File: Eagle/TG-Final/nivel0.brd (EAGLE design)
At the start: 21 parts

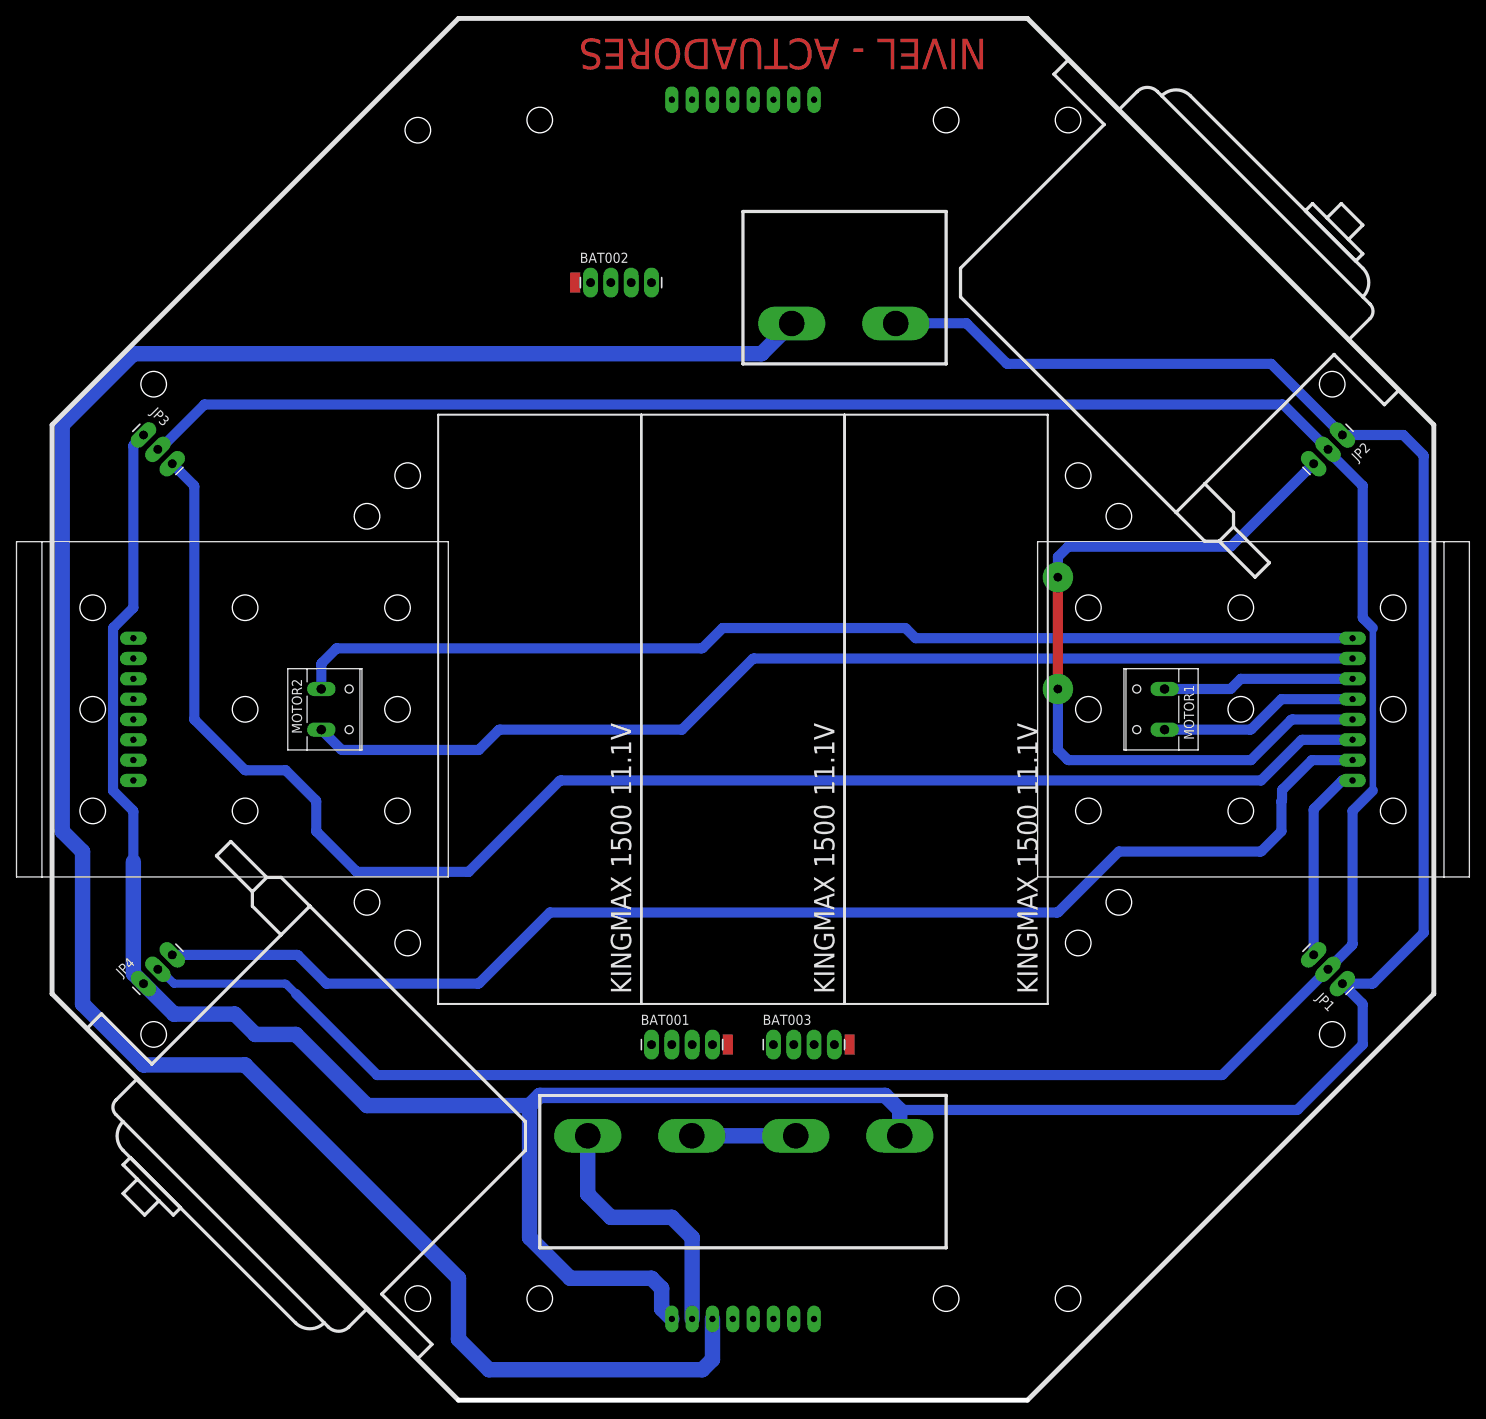
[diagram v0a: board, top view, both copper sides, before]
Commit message: Routing placa Actuadores. Listo??
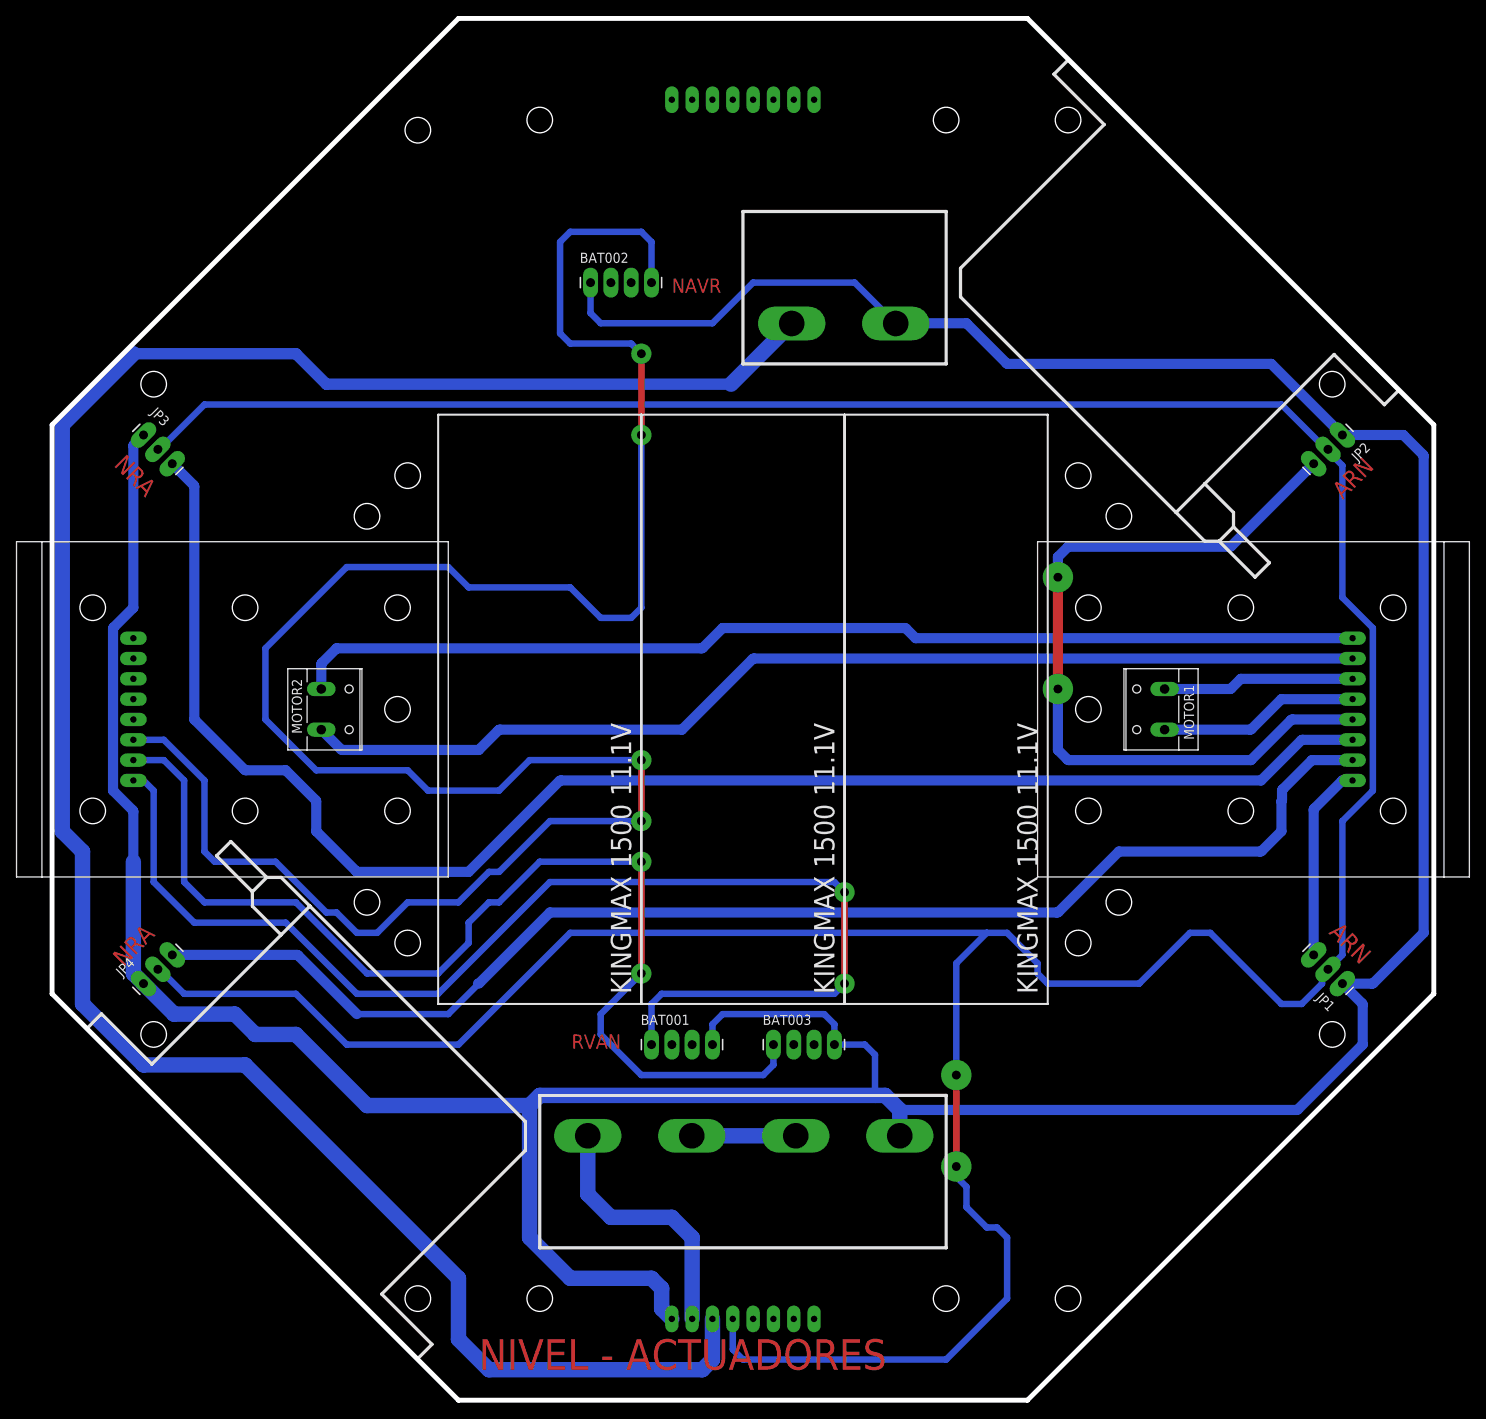
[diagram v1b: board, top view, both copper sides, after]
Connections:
- removed net +6V: JP1.2, JP2.2, JP3.2, JP4.2
- new net P$1: JP1.2, JP2.2, JP3.2, JP4.2, U$1.PIN19
- new net SENSE1: BAT001.1, U$1.PIN15
- new net SENSE2: BAT002.4, U$1.PIN13
- new net SENSE3: BAT003.1, U$1.PIN14
- net VSS: now also BAT001.4, BAT002.1, BAT003.4
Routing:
- net P$1: track 0.00 -> 481.1 mm, vias 0 -> 2
- net +6V: track 377.6 -> 0.00 mm
- net SENSE2: track 0.00 -> 279.6 mm, vias 0 -> 4
- net SENSE1: track 0.00 -> 154.6 mm, vias 0 -> 2
- net SENSE3: track 0.00 -> 139.7 mm, vias 0 -> 2
- net VSS: track 432.2 -> 511.0 mm
- net +12V: track 277.6 -> 281.0 mm
- net SERVO04: track 163.5 -> 166.7 mm
- added copper zone on layer 16, net N$2
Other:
- board outline added: 172.7 x 172.7 mm
- board text added: "ARN"
- board text added: "NAVR"
- board text added: "NRA"
- board text added: "RVAN"

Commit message: Mejoras en placa de Actuadores y otros
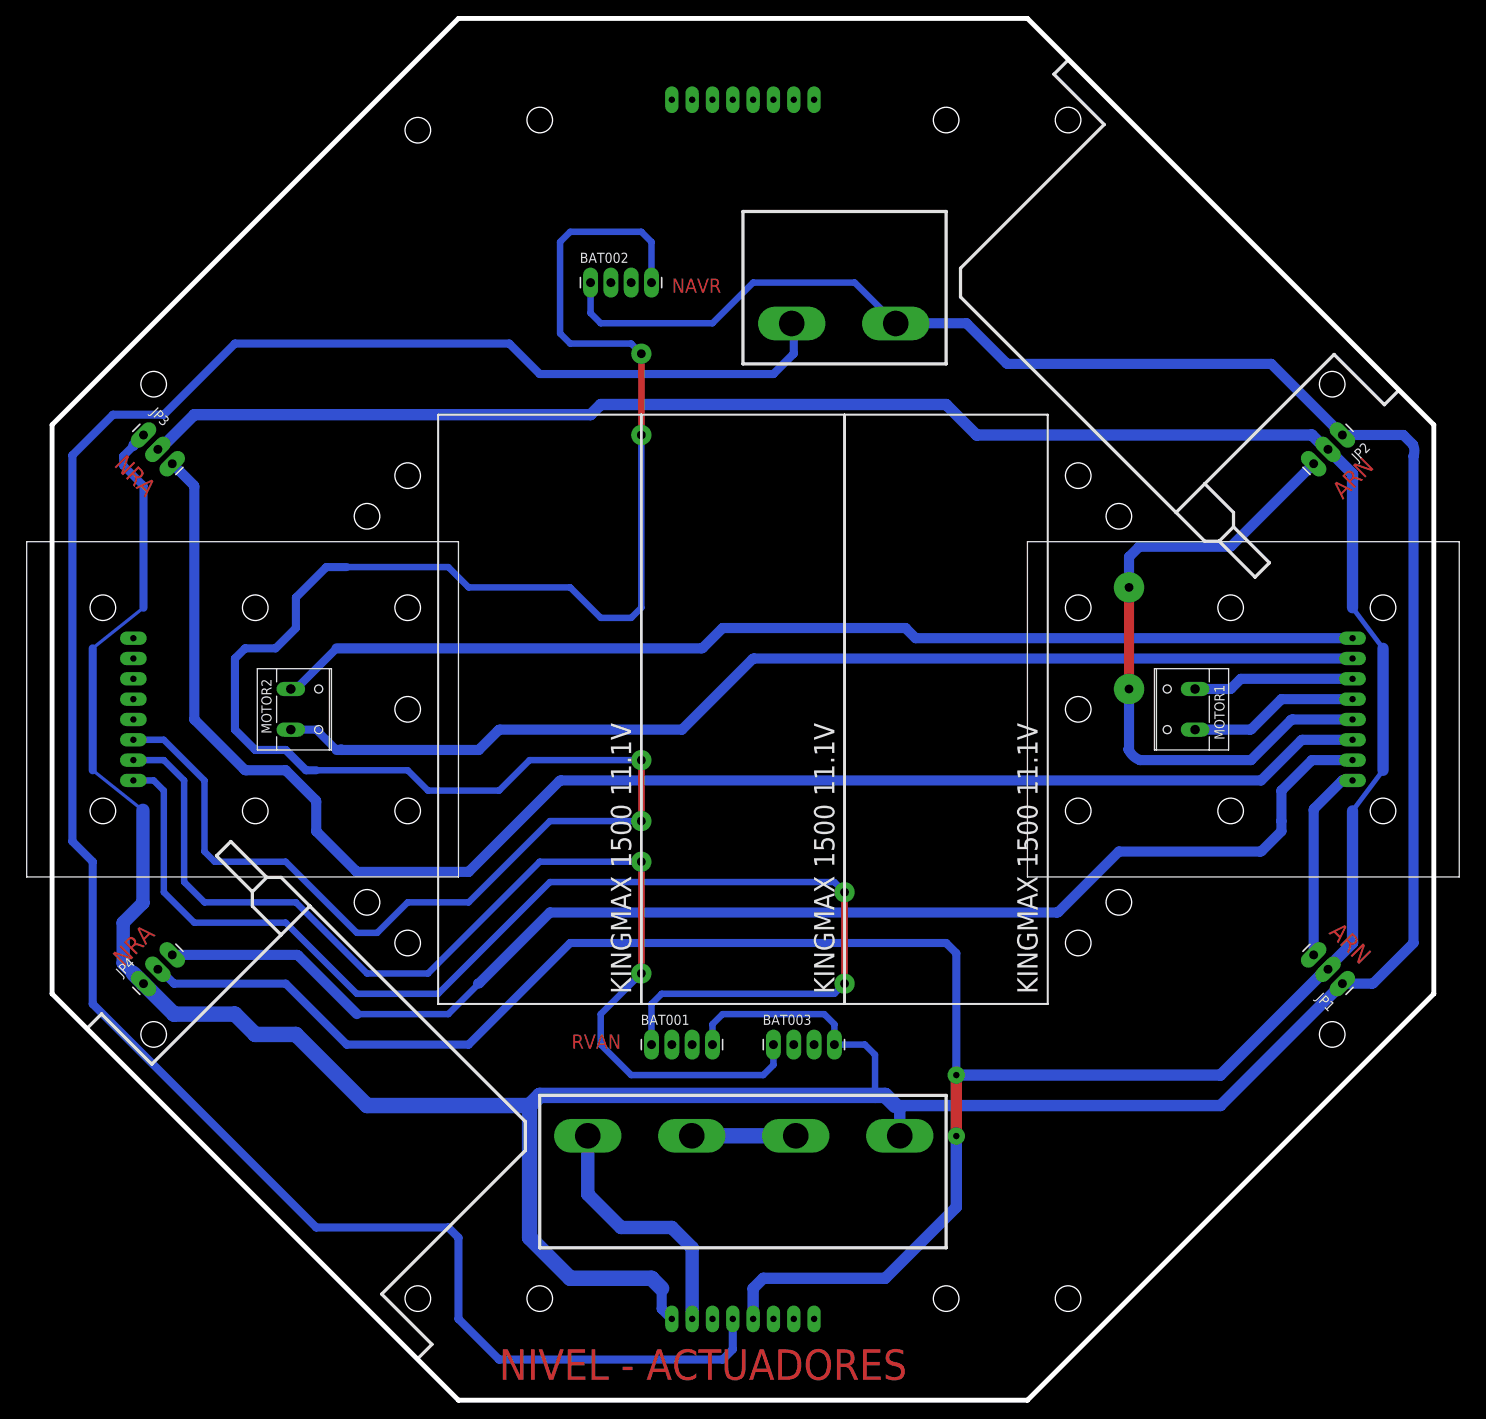
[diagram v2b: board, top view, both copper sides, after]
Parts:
- moved MOTOR2 3.81 mm to (-156.2, 87.6)
- moved MOTOR1 3.81 mm to (-44.5, 87.6)
- moved U$5 1.27 mm to (-161.3, 87.6)
- moved U$6 1.27 mm to (-39.4, 87.6)
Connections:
- net +24V renamed +22V
- removed net P$1: JP1.2, JP2.2, JP3.2, JP4.2, U$1.PIN19
- new net +11V1: U$1.PIN19, U$12.P$2
- new net +6V: JP1.2, JP2.2, JP3.2, JP4.2, U$1.PIN20
- net +12V: no longer U$12.P$2
- net +3V3: now also U$1.PIN22; no longer U$1.PIN21
- net +5V: now also U$1.PIN21; no longer U$1.PIN20
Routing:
- net P$1: track 481.1 -> 0.00 mm, vias 2 -> 0
- net +6V: track 0.00 -> 447.6 mm, vias 0 -> 2
- net +12V: track 281.0 -> 0.00 mm
- net +11V1: track 0.00 -> 280.7 mm
- net SERVO02: track 100.3 -> 82.8 mm
- net SENSE2: track 279.6 -> 289.4 mm
- net M2-RED: track 134.6 -> 138.7 mm
- net M1-BLACK: track 25.1 -> 21.2 mm
- net M1-RED: track 24.0 -> 20.2 mm
- net M2-BLACK: track 134.4 -> 136.4 mm
- net SENSE1: track 154.6 -> 155.4 mm
- net SENSE3: track 139.7 -> 139.0 mm
- net +22V: track 32.8 -> 32.0 mm
